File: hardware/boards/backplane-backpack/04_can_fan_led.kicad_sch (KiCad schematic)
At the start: 22 parts, among them J2 CANH/CANL/GND (TBD), J9 12V FAN (TBD), Q1 AO3407A, Q2 2N7002,215, U3 TCAN3413DR

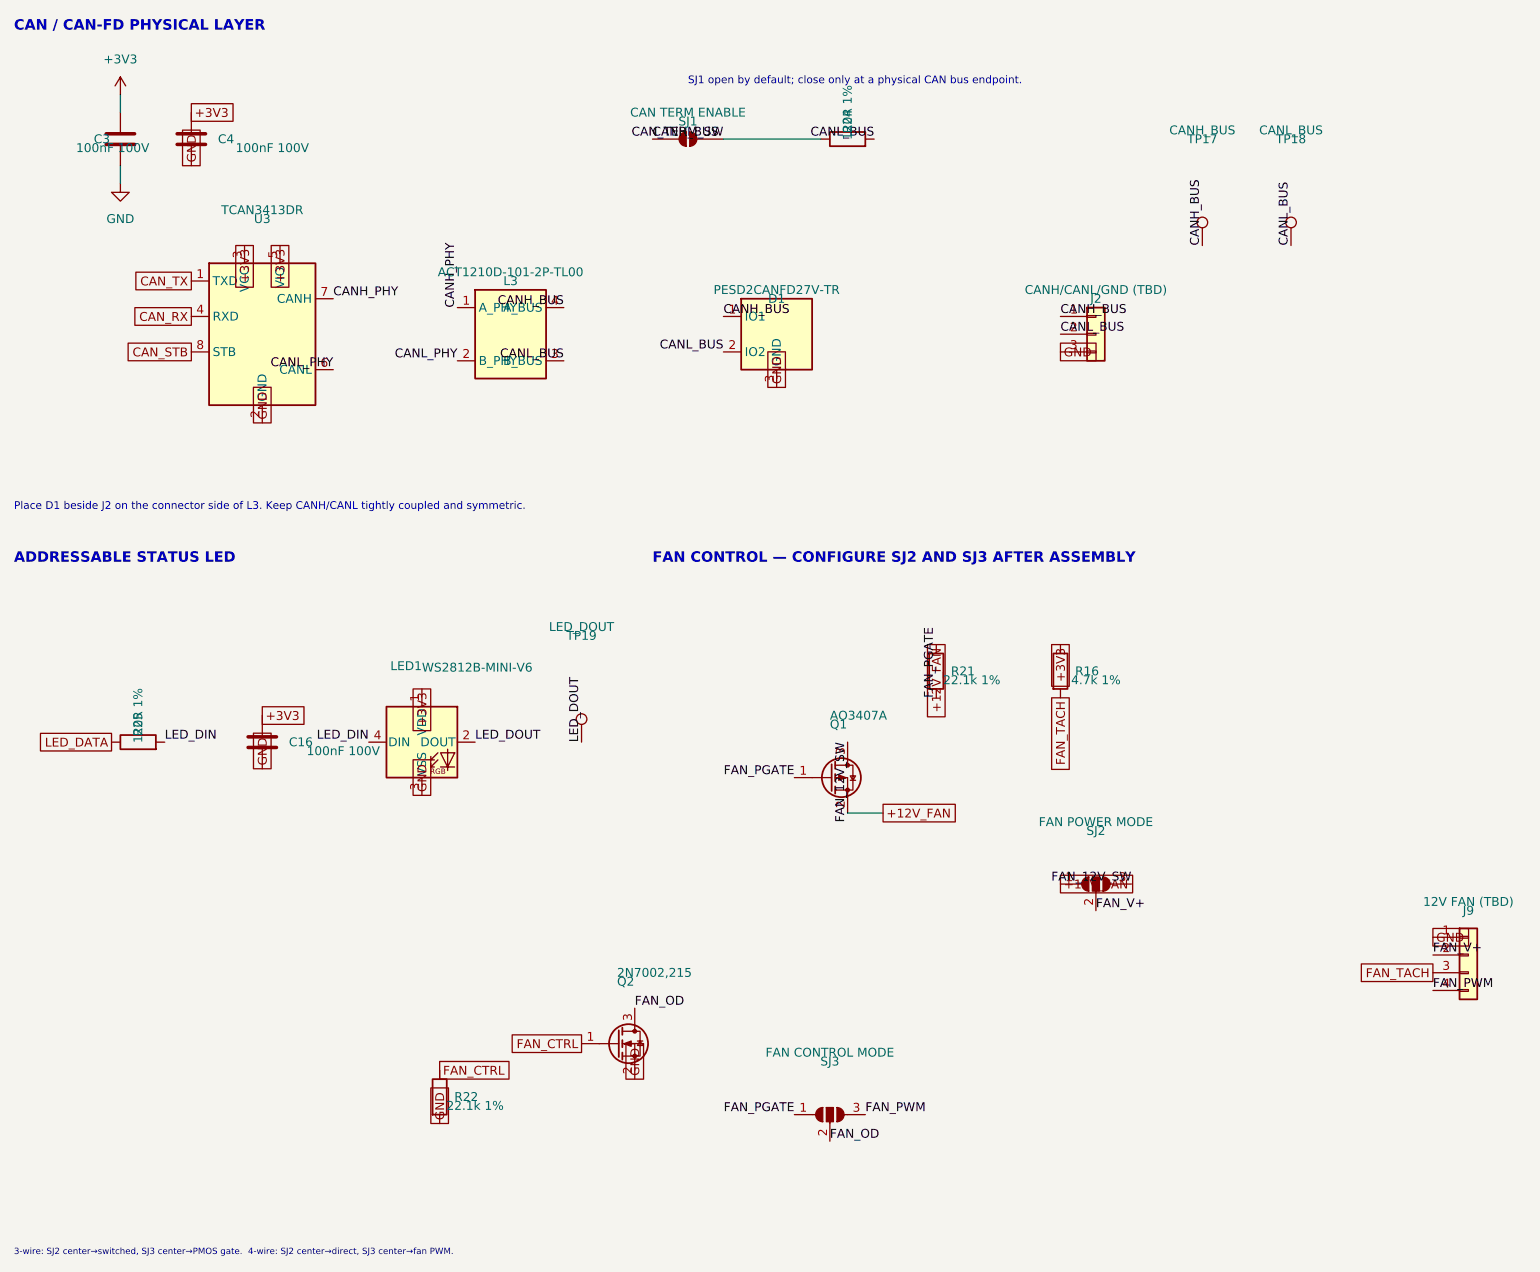
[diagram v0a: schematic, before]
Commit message: chore: checkpoint workspace changes
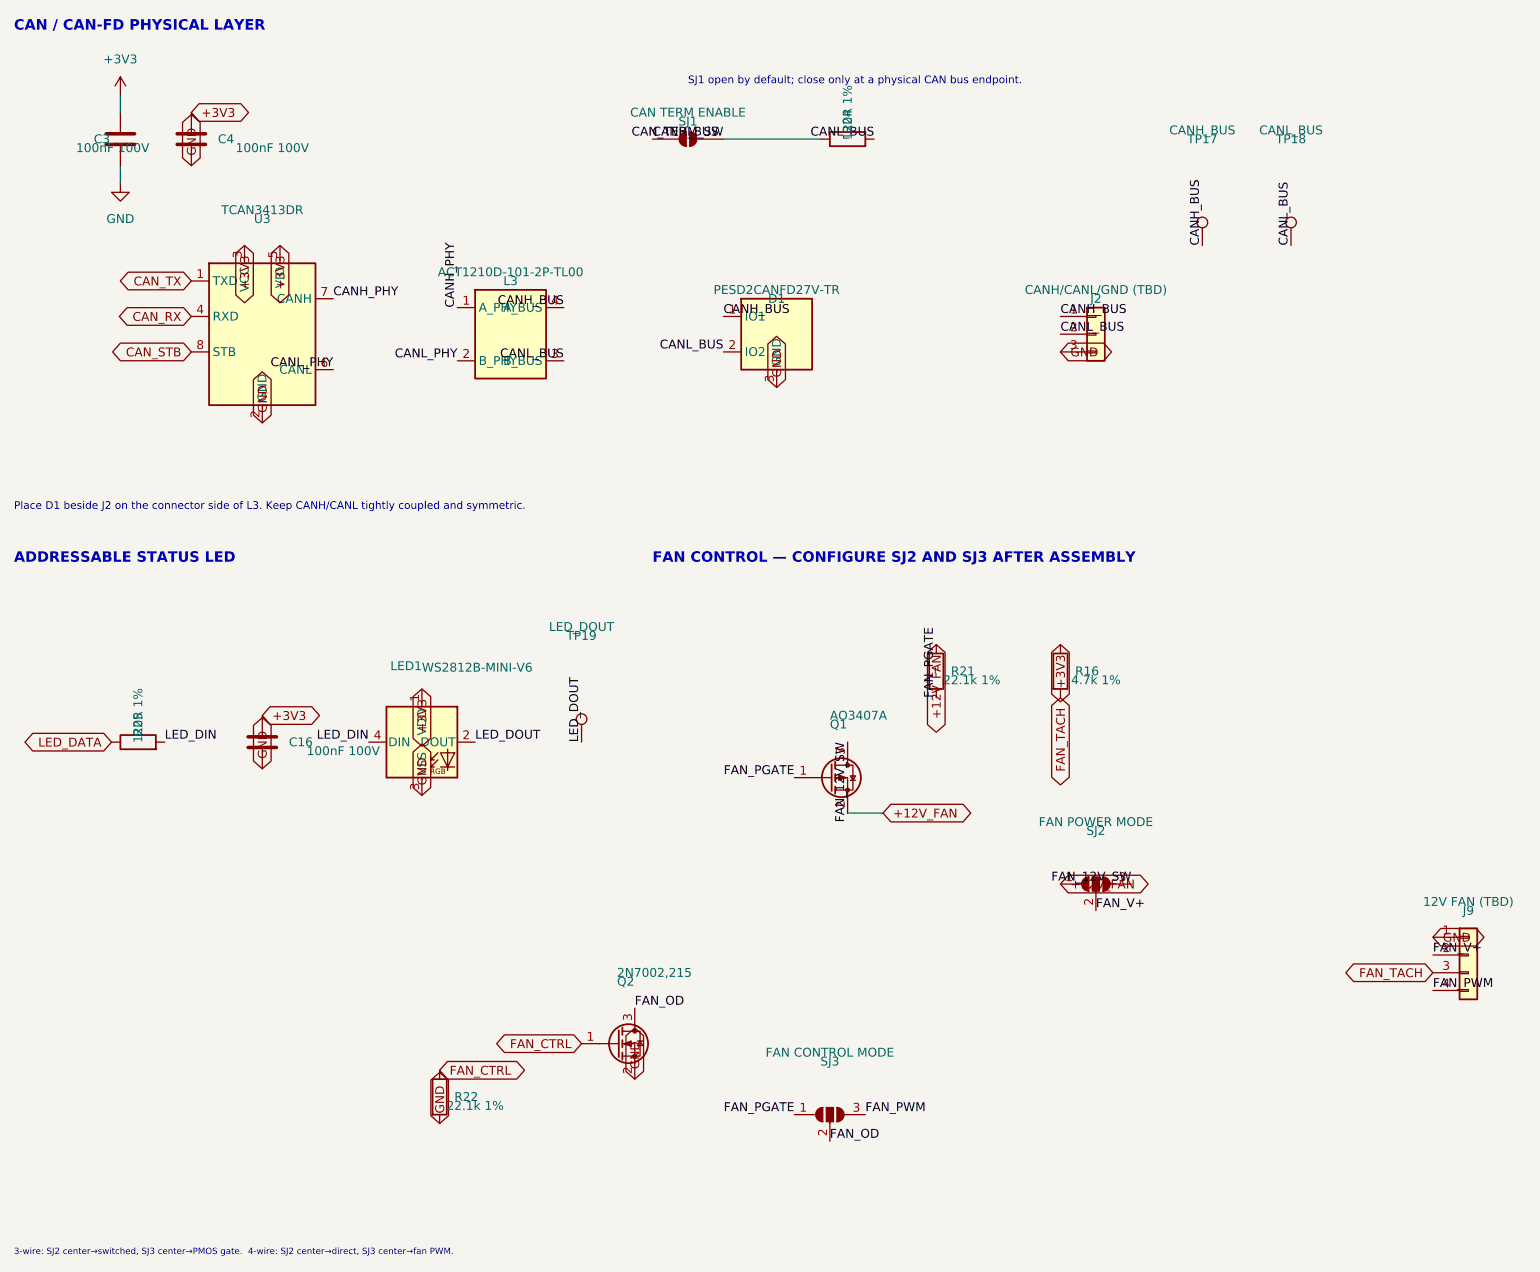
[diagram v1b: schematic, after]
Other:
- company: (none) -> Karl Quinsland
- title: CAN Fan and Status -> Backplane Backpack
